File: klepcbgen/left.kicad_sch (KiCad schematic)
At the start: 58 parts, among them K0 Esc, K1 !,1,,F1, K15 Tab, K16 Q, K17 W, K18 E, K19 R, K2 @,2,,F2, K20 T, K3 #,3,,F3, K30 Caps Lock, K31 A, K32 S, K33 D, K34 F, K35 G, K4 $,4,,F4, K44 Shift, K45 Z, K46 X, K47 C, K48 V, K49 B, K5 %,5,,F5, K58 Ctrl, K59 Win, K6 ^,6,,F6, K60 Alt, K61 Space

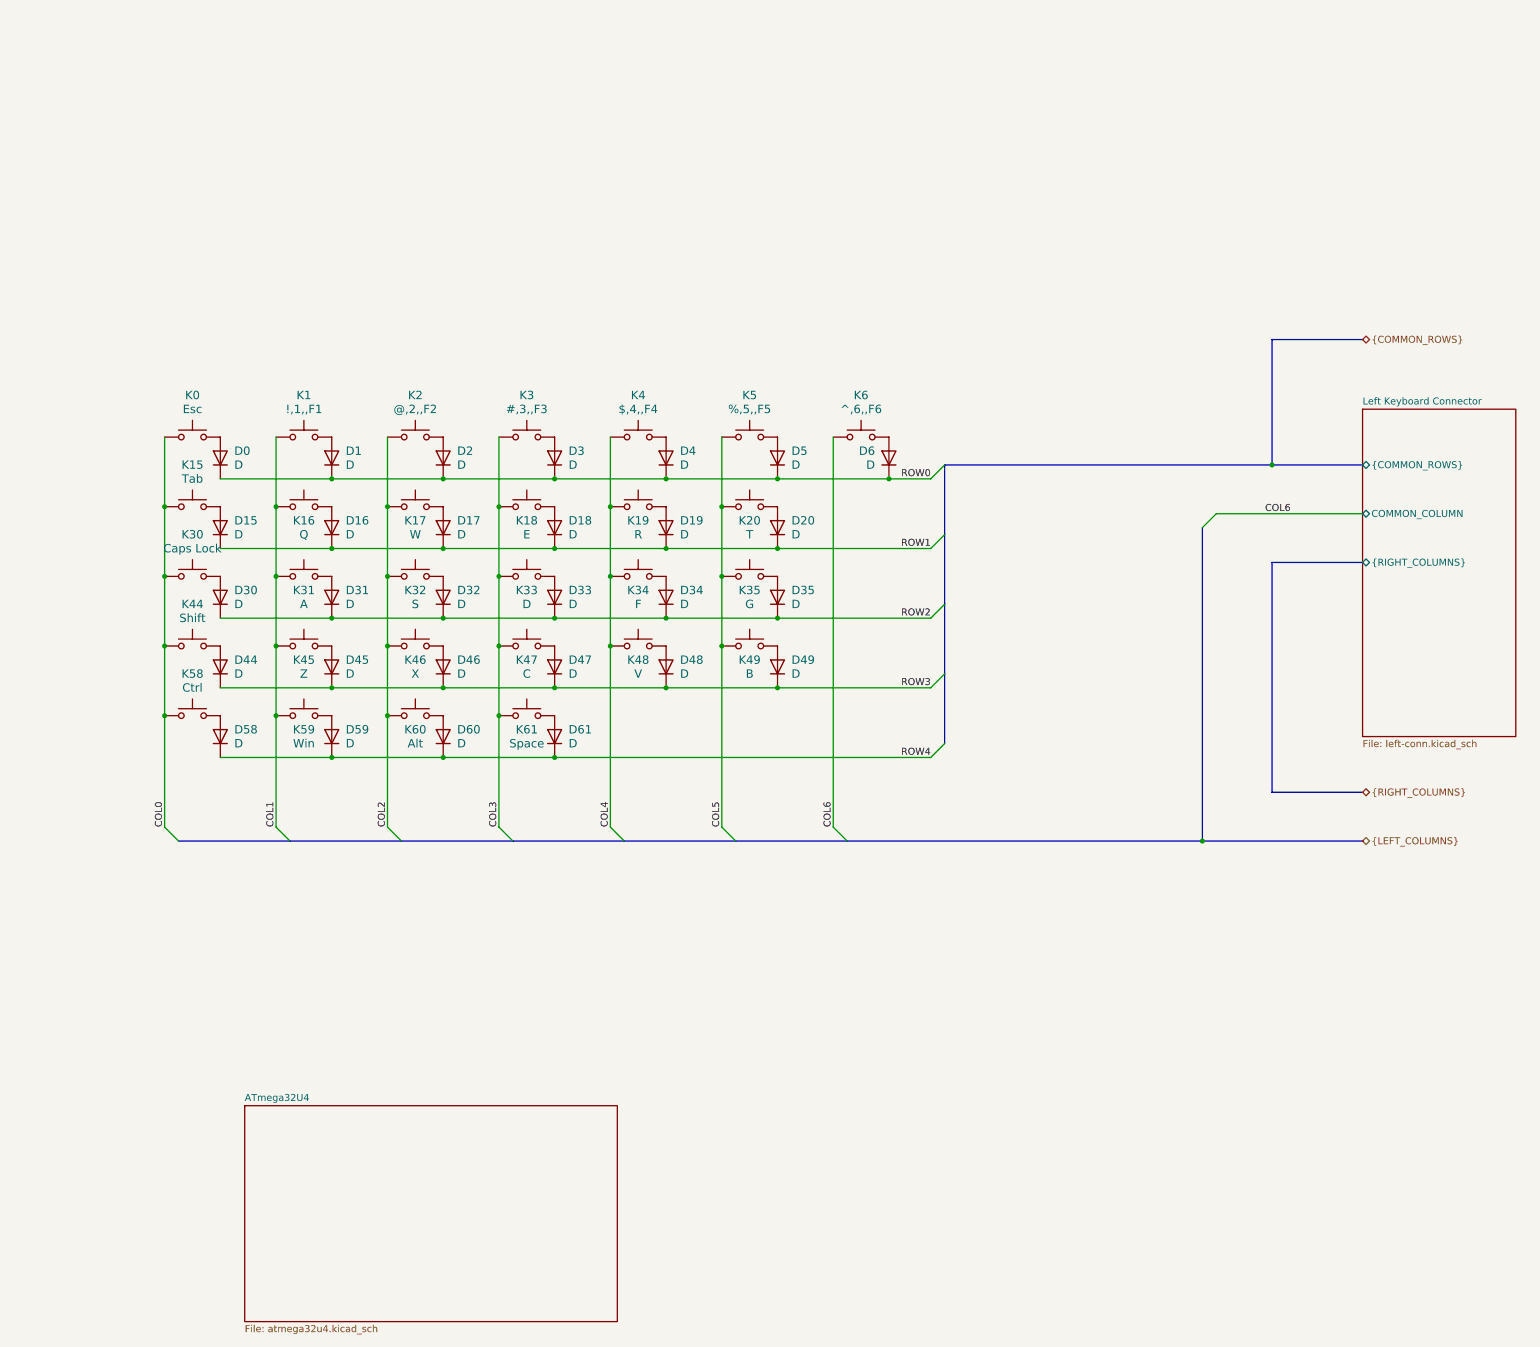
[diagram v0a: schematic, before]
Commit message: Continuing.
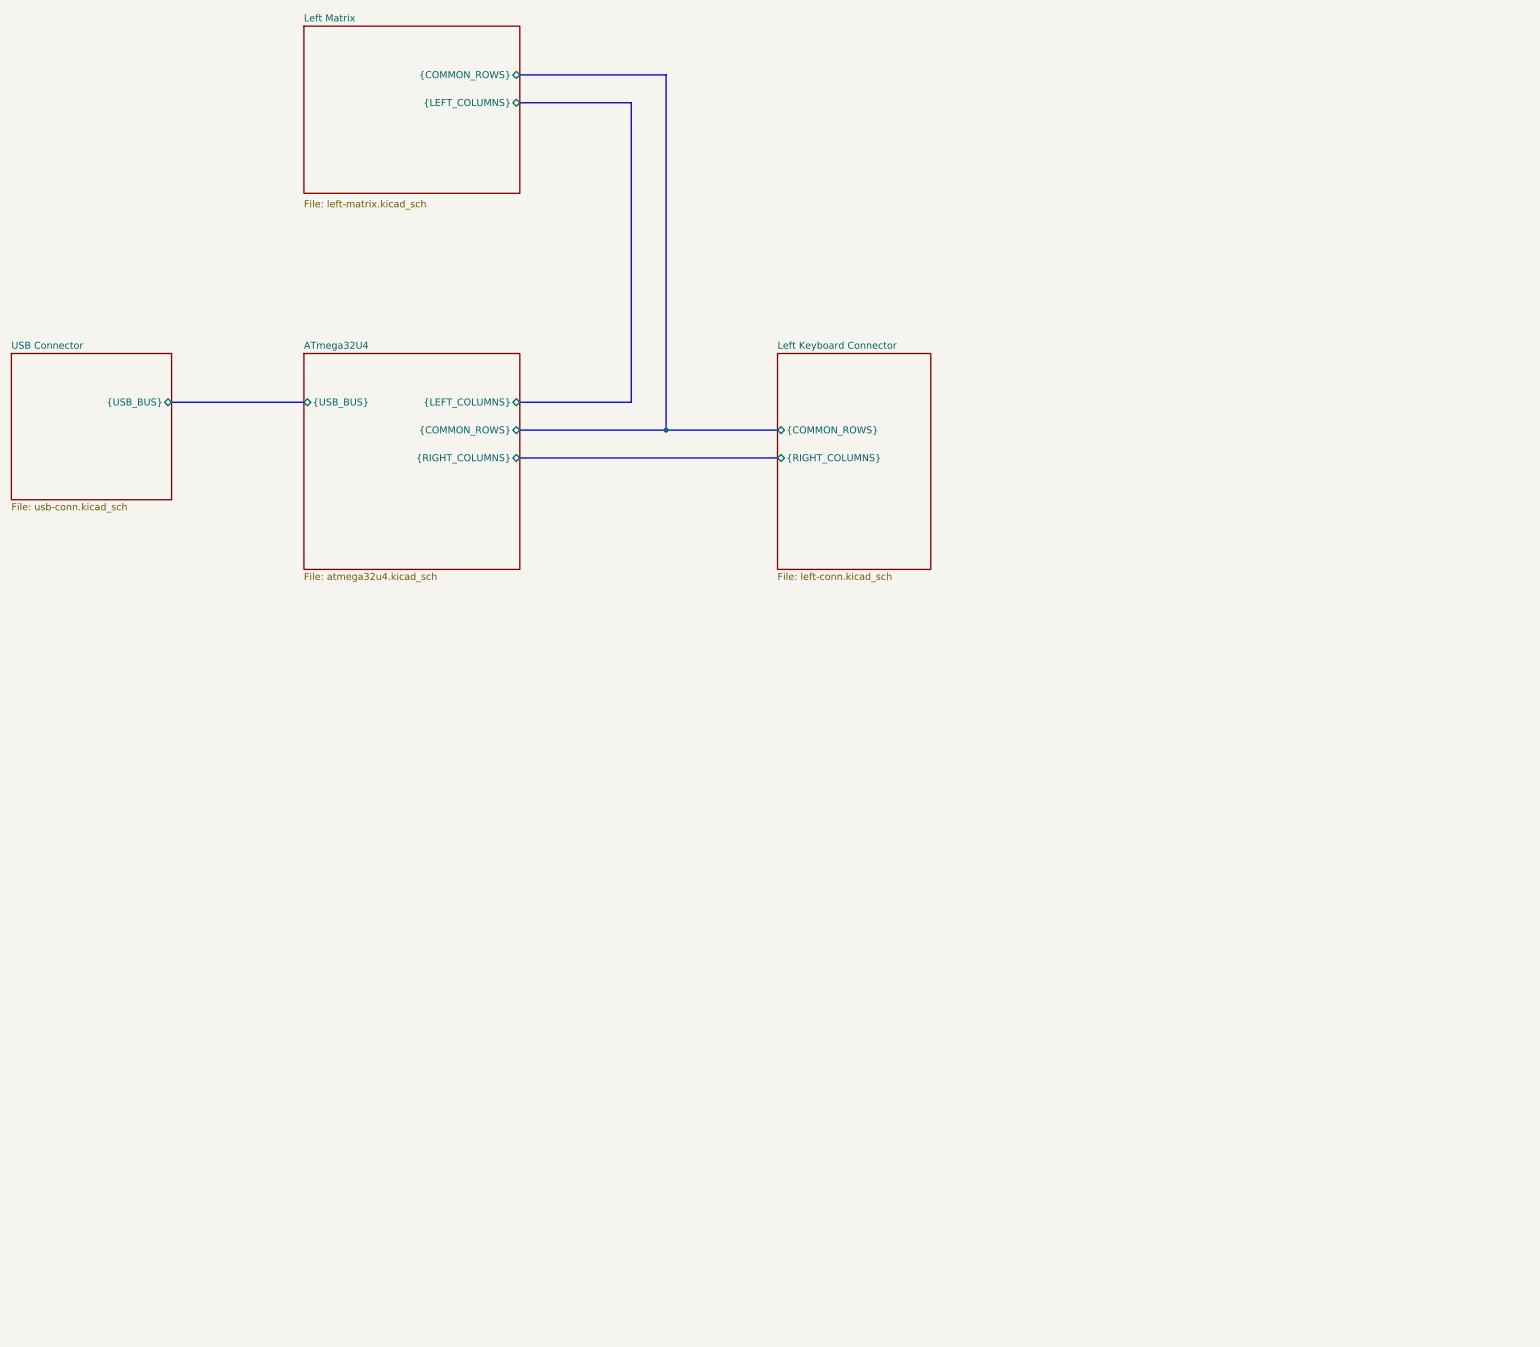
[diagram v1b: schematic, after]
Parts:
- removed D0, D1, D15, D16, D17, D18, D19, D2, D20, D3, D30, D31, D32, D33, D34, D35, D4, D44, D45, D46, D47, D48, D49, D5, D58, D59, D6, D60, D61: D, Diode_SMD:D_0805_2012Metric_Pad1.15x1.40mm_HandSolder, symbol Device:D
- removed K0: Esc, Button_Switch_Keyboard:SW_Cherry_MX_1.00u_PCB, symbol Switch:SW_Push
- removed K1: !,1,,F1, Button_Switch_Keyboard:SW_Cherry_MX_1.00u_PCB, symbol Switch:SW_Push
- removed K15: Tab, Button_Switch_Keyboard:SW_Cherry_MX_1.50u_PCB, symbol Switch:SW_Push
- removed K16: Q, Button_Switch_Keyboard:SW_Cherry_MX_1.00u_PCB, symbol Switch:SW_Push
- removed K17: W, Button_Switch_Keyboard:SW_Cherry_MX_1.00u_PCB, symbol Switch:SW_Push
- removed K18: E, Button_Switch_Keyboard:SW_Cherry_MX_1.00u_PCB, symbol Switch:SW_Push
- removed K19: R, Button_Switch_Keyboard:SW_Cherry_MX_1.00u_PCB, symbol Switch:SW_Push
- removed K2: @,2,,F2, Button_Switch_Keyboard:SW_Cherry_MX_1.00u_PCB, symbol Switch:SW_Push
- removed K20: T, Button_Switch_Keyboard:SW_Cherry_MX_1.00u_PCB, symbol Switch:SW_Push
- removed K3: #,3,,F3, Button_Switch_Keyboard:SW_Cherry_MX_1.00u_PCB, symbol Switch:SW_Push
- removed K30: Caps Lock, Button_Switch_Keyboard:SW_Cherry_MX_1.75u_PCB, symbol Switch:SW_Push
- removed K31: A, Button_Switch_Keyboard:SW_Cherry_MX_1.00u_PCB, symbol Switch:SW_Push
- removed K32: S, Button_Switch_Keyboard:SW_Cherry_MX_1.00u_PCB, symbol Switch:SW_Push
- removed K33: D, Button_Switch_Keyboard:SW_Cherry_MX_1.00u_PCB, symbol Switch:SW_Push
- removed K34: F, Button_Switch_Keyboard:SW_Cherry_MX_1.00u_PCB, symbol Switch:SW_Push
- removed K35: G, Button_Switch_Keyboard:SW_Cherry_MX_1.00u_PCB, symbol Switch:SW_Push
- removed K4: $,4,,F4, Button_Switch_Keyboard:SW_Cherry_MX_1.00u_PCB, symbol Switch:SW_Push
- removed K44: Shift, Button_Switch_Keyboard:SW_Cherry_MX_2.25u_PCB, symbol Switch:SW_Push
- removed K45: Z, Button_Switch_Keyboard:SW_Cherry_MX_1.00u_PCB, symbol Switch:SW_Push
- removed K46: X, Button_Switch_Keyboard:SW_Cherry_MX_1.00u_PCB, symbol Switch:SW_Push
- removed K47: C, Button_Switch_Keyboard:SW_Cherry_MX_1.00u_PCB, symbol Switch:SW_Push
- removed K48: V, Button_Switch_Keyboard:SW_Cherry_MX_1.00u_PCB, symbol Switch:SW_Push
- removed K49: B, Button_Switch_Keyboard:SW_Cherry_MX_1.00u_PCB, symbol Switch:SW_Push
- removed K5: %,5,,F5, Button_Switch_Keyboard:SW_Cherry_MX_1.00u_PCB, symbol Switch:SW_Push
- removed K58: Ctrl, Button_Switch_Keyboard:SW_Cherry_MX_1.25u_PCB, symbol Switch:SW_Push
- removed K59: Win, Button_Switch_Keyboard:SW_Cherry_MX_1.25u_PCB, symbol Switch:SW_Push
- removed K6: ^,6,,F6, Button_Switch_Keyboard:SW_Cherry_MX_1.00u_PCB, symbol Switch:SW_Push
- removed K60: Alt, Button_Switch_Keyboard:SW_Cherry_MX_1.25u_PCB, symbol Switch:SW_Push
- removed K61: Space, Button_Switch_Keyboard:SW_Cherry_MX_2.75u_PCB, symbol Switch:SW_Push
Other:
- added sheet Left Matrix (left-matrix.kicad_sch)
- added sheet USB Connector (usb-conn.kicad_sch)
- sheet ATmega32U4 ports: added {COMMON_ROWS}, {LEFT_COLUMNS}, {RIGHT_COLUMNS}, {USB_BUS}; removed none
- sheet Left Keyboard Connector ports: added none; removed COMMON_COLUMN
